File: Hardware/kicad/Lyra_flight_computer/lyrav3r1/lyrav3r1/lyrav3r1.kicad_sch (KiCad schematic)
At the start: 77 parts, among them J1 Conn_01x02, J2 Screw_Terminal_01x06, J3 Conn_01x02, J4 Conn_01x02, J6 Conn_01x06, J7 USB_B_Micro, J8 Conn_01x04, J9 Screw_Terminal_01x06, Q1 AO3401A, Q2 AO3400A, Q3 AO3400A, Q4 AO3400A, Q5 AO3400A, U1 STM32WLE5CBUx, U2 BMI088, U3 BMP388, U4 ADXL375BCCZ-RL7, U5 AMS1117-3.3, U8 RP2040, U9 W25Q128JVS, X2 SX1M12.000M10F30TNN

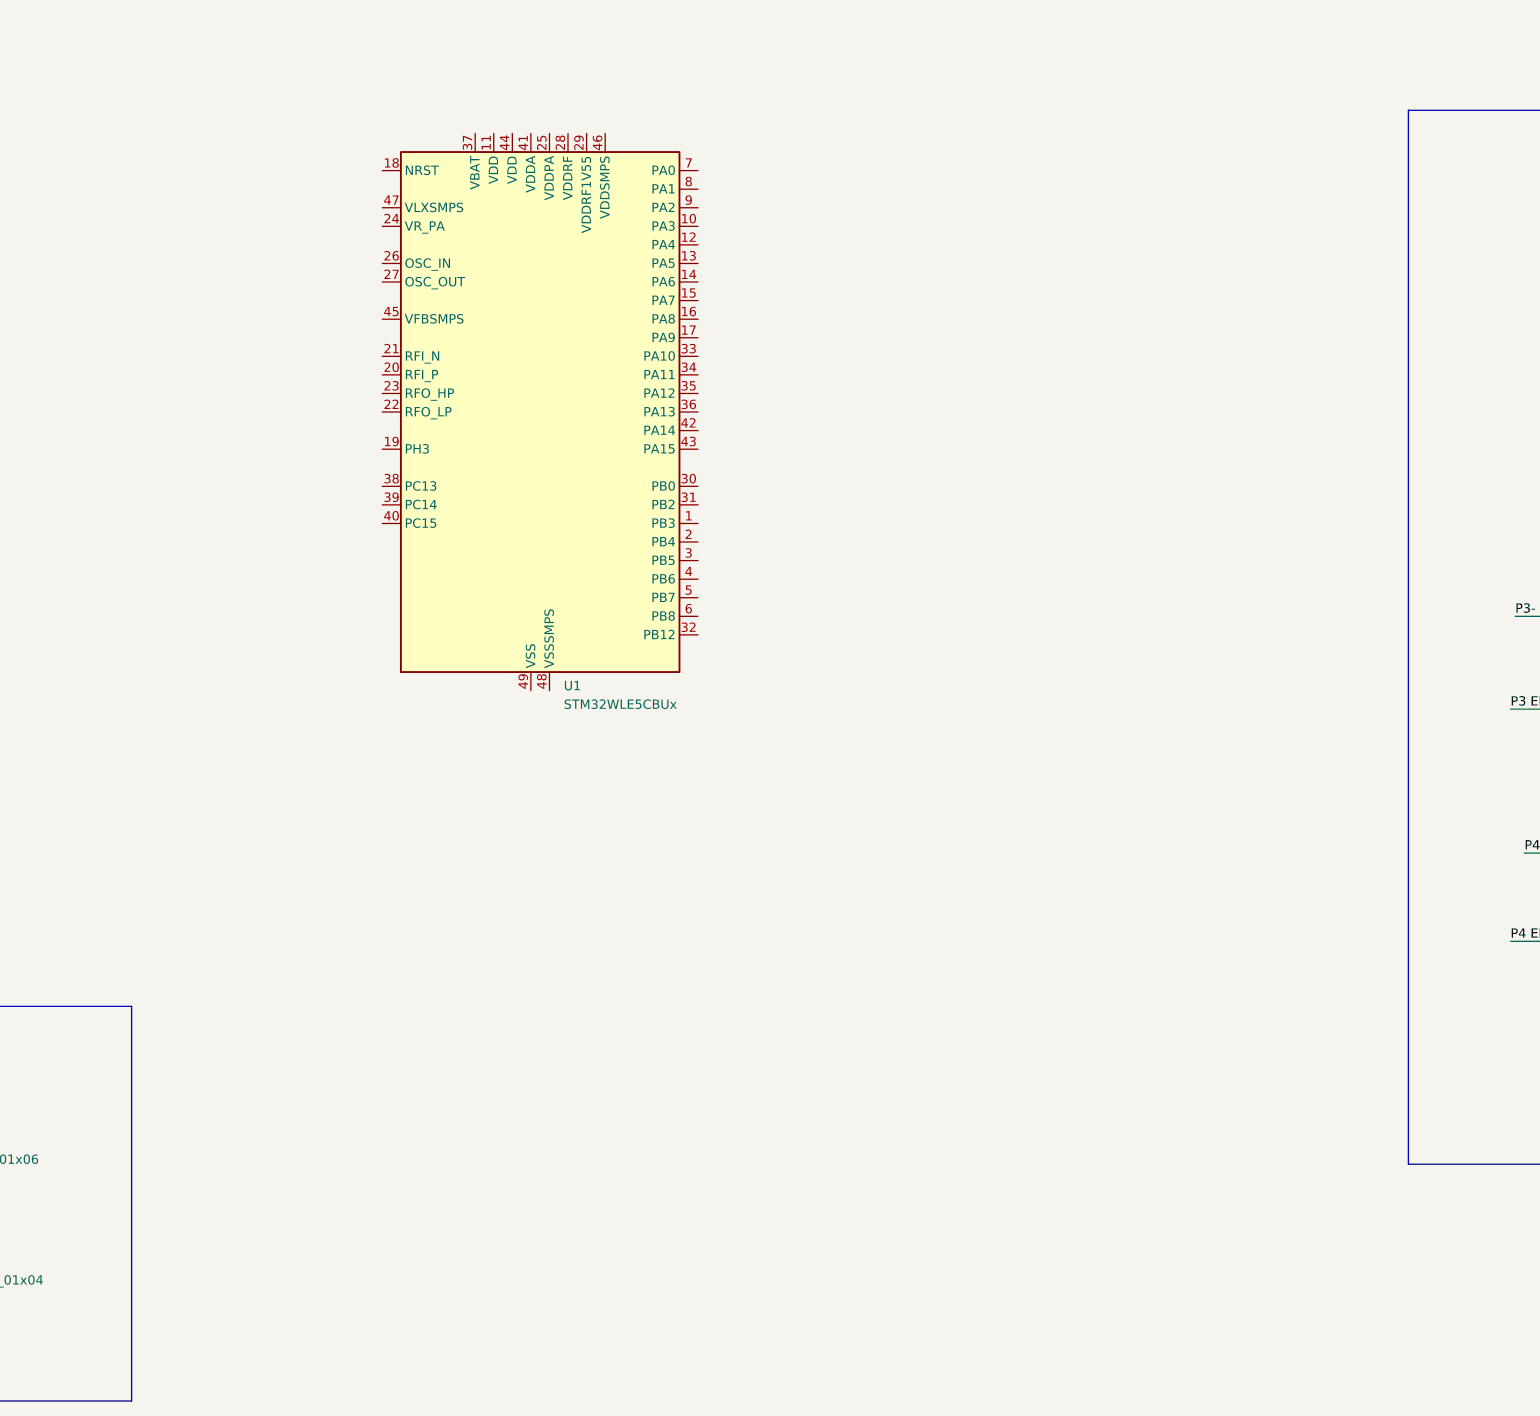
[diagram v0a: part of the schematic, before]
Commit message: stuffs
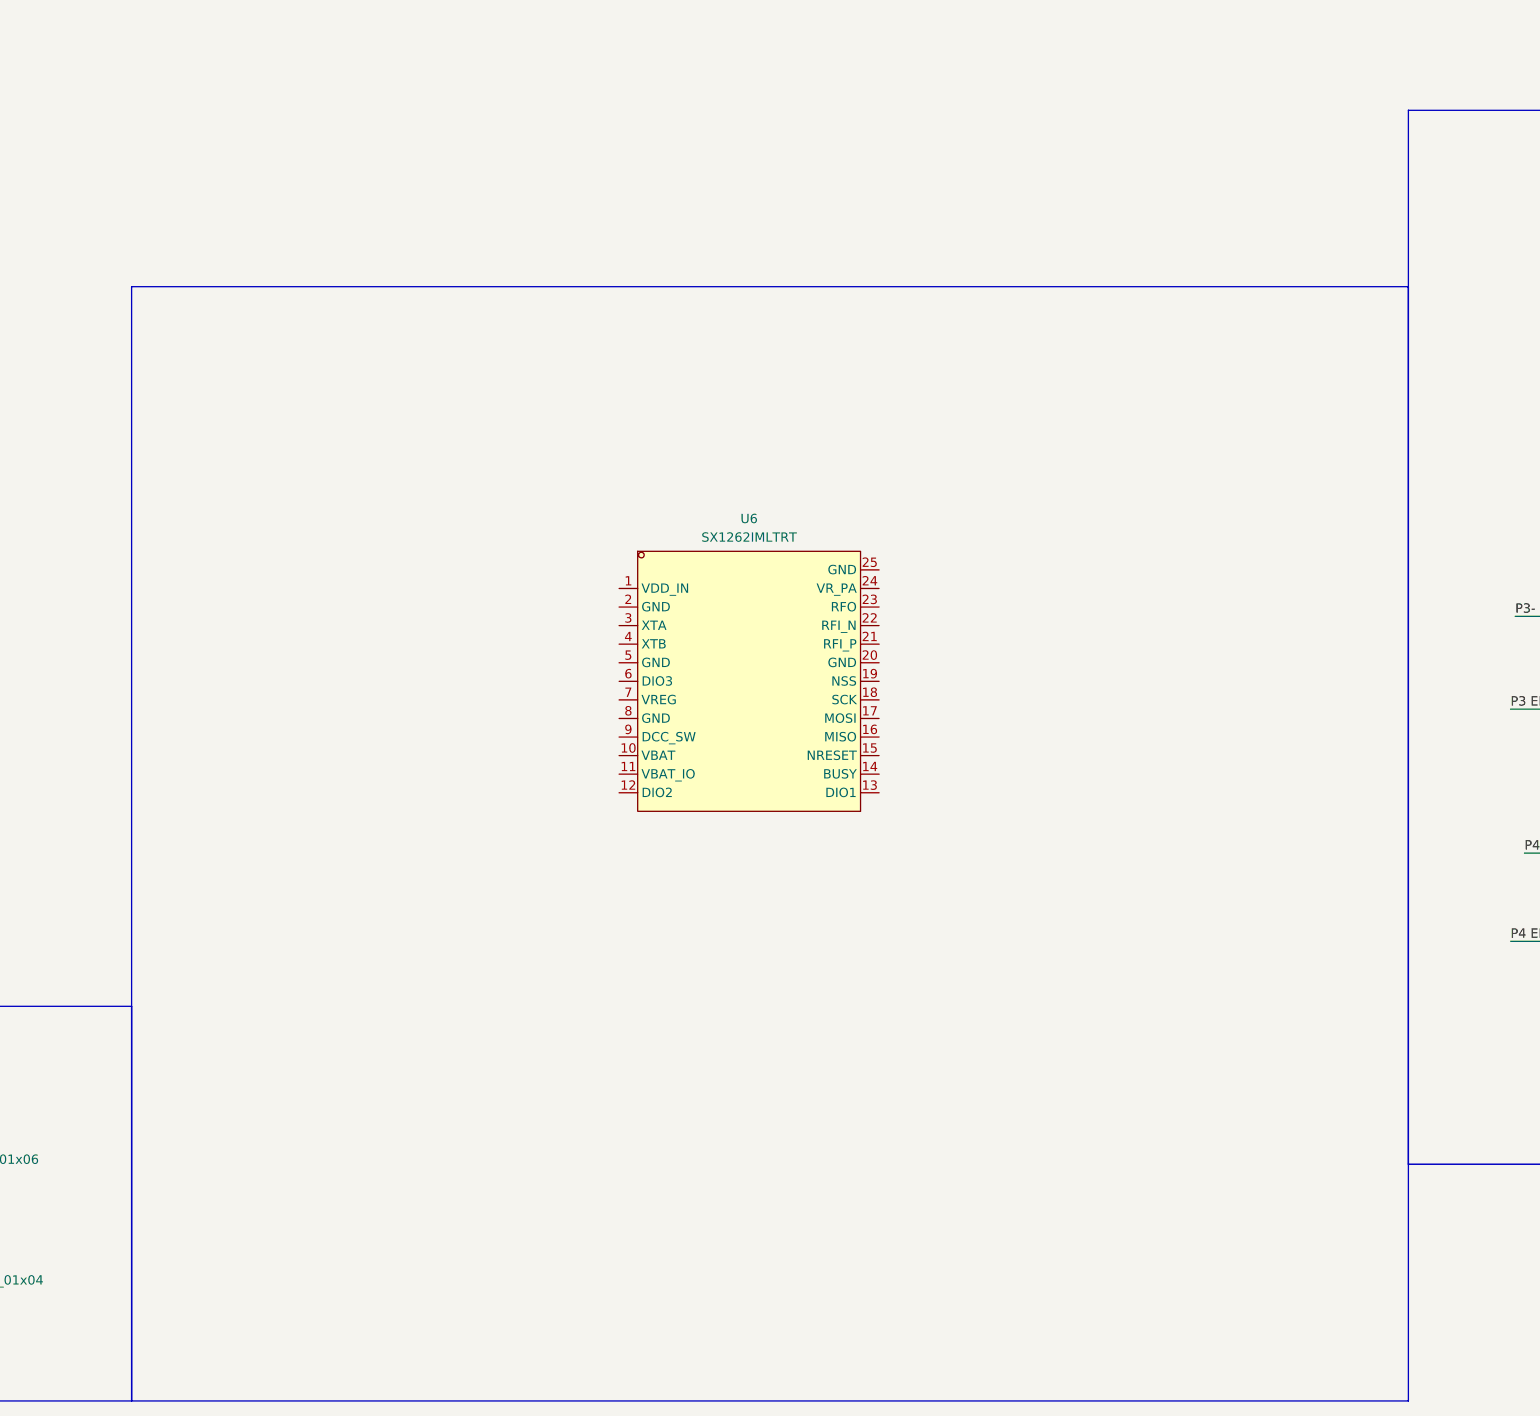
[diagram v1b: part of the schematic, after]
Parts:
- removed U1: STM32WLE5CBUx, Package_DFN_QFN:QFN-48-1EP_7x7mm_P0.5mm_EP5.6x5.6mm, symbol MCU_ST_STM32WL:STM32WLE5CBUx
- added U6: SX1262IMLTRT, easyeda2kicad:QFN-24_L4.0-W4.0-P0.50-BL-EP2.6, symbol easyeda2kicad:SX1262IMLTRT
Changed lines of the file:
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@@
     (fill (type none))
   )
+  (rectangle (start 299.72 255.905) (end 474.345 408.305)
+    (stroke (width 0) (type default))
+    (fill (type none))
+  )
   (rectangle (start 283.845 12.7) (end 407.035 70.485)
     (stroke (width 0) (type default))
@@
     )
   )
+  (symbol (lib_id "easyeda2kicad:SX1262IMLTRT") (at 384.175 309.88 0) (unit 1)
+    (in_bom yes) (on_board yes) (dnp no) (fields_autoplaced)
+    (property "Reference" "U6" (at 384.175 287.655 0)
+      (effects (font (size 1.27 1.27)))
+    )
+    (property "Value" "SX1262IMLTRT" (at 384.175 290.195 0)
+      (effects (font (size 1.27 1.27)))
+    )
+    (property "Footprint" "easyeda2kicad:QFN-24_L4.0-W4.0-P0.50-BL-EP2.6" (at 384.175 332.74 0)
+      (effects (font (size 1.27 1.27)) hide)
+    )
+    (property "Datasheet" "https://lcsc.com/product-detail/Others_STMicroelectronics_SX1262IMLTRT_STMicroelectronics-SX1262IMLTRT_C191341.html" (at 384.175 335.28 0)
+      (effects (font (size 1.27 1.27)) hide)
+    )
+    (property "LCSC Part" "C191341" (at 384.175 337.82 0)
+      (effects (font (size 1.27 1.27)) hide)
+    )
+    (pin "1")
+    (pin "10")
+    (pin "11")
+    (pin "12")
+    (pin "13")
+    (pin "14")
+    (pin "15")
+    (pin "16")
+    (pin "17")
+    (pin "18")
+    (pin "19")
+    (pin "2")
+    (pin "20")
+    (pin "21")
+    (pin "22")
+    (pin "23")
+    (pin "24")
+    (pin "25")
+    (pin "3")
+    (pin "4")
+    (pin "5")
+    (pin "6")
+    (pin "7")
+    (pin "8")
+    (pin "9")
+    (instances
+      (project "lyrav3r1"
+        (path "/12cc3c39-e34e-4801-bd3f-38f875d59424"
+          (reference "U6") (unit 1)
+        )
+      )
+    )
+  )
   (symbol (lib_id "power:GND") (at 554.99 322.58 0) (unit 1)
     (in_bom yes) (on_board yes) (dnp no) (fields_autoplaced)
@@
         )
       )
-    )
-  )
-  (symbol (lib_id "MCU_ST_STM32WL:STM32WLE5CBUx") (at 354.33 273.05 0) (unit 1)
-    (in_bom yes) (on_board yes) (dnp no) (fields_autoplaced)
-    (property "Reference" "U1" (at 358.8259 310.515 0)
-      (effects (font (size 1.27 1.27)) (justify left))
-    )
-    (property "Value" "STM32WLE5CBUx" (at 358.8259 313.055 0)
-      (effects (font (size 1.27 1.27)) (justify left))
-    )
-    (property "Footprint" "Package_DFN_QFN:QFN-48-1EP_7x7mm_P0.5mm_EP5.6x5.6mm" (at 336.55 308.61 0)
-      (effects (font (size 1.27 1.27)) (justify right) hide)
-    )
-    (property "Datasheet" "https://www.st.com/resource/en/datasheet/stm32wle5cb.pdf" (at 354.33 273.05 0)
-      (effects (font (size 1.27 1.27)) hide)
-    )
-    (pin "1")
-    (pin "10")
-    (pin "11")
-    (pin "12")
-    (pin "13")
-    (pin "14")
-    (pin "15")
-    (pin "16")
-    (pin "17")
-    (pin "18")
-    (pin "19")
-    (pin "2")
-    (pin "20")
-    (pin "21")
-    (pin "22")
-    (pin "23")
-    (pin "24")
-    (pin "25")
-    (pin "26")
-    (pin "27")
-    (pin "28")
-    (pin "29")
-    (pin "3")
-    (pin "30")
-    (pin "31")
-    (pin "32")
-    (pin "33")
-    (pin "34")
-    (pin "35")
-    (pin "36")
-    (pin "37")
-    (pin "38")
-    (pin "39")
-    (pin "4")
-    (pin "40")
-    (pin "41")
-    (pin "42")
-    (pin "43")
-    (pin "44")
-    (pin "45")
-    (pin "46")
-    (pin "47")
-    (pin "48")
-    (pin "49")
-    (pin "5")
-    (pin "6")
-    (pin "7")
-    (pin "8")
-    (pin "9")
-    (instances
-      (project "lyrav3r1"
-        (path "/12cc3c39-e34e-4801-bd3f-38f875d59424"
-          (reference "U1") (unit 1)
-        )
-      )

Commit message: asd
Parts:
- removed J6: Conn_01x06, Connector_PinHeader_2.54mm:PinHeader_1x06_P2.54mm_Vertical, symbol Connector_Generic:Conn_01x06
- removed J8: Conn_01x04, Connector_PinHeader_2.54mm:PinHeader_1x04_P2.54mm_Vertical, symbol Connector_Generic:Conn_01x04
- added D3: D, symbol Device:D
- added J5: Conn_01x05, symbol Connector_Generic:Conn_01x05
- added R8: 100, Resistor_SMD:R_0402_1005Metric, symbol Device:R_Small
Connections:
- net BRKOUT1: now also J5.1 (Pin_1)
- net BRKOUT2: now also J5.2 (Pin_2)
- net BRKOUT3: now also J5.3 (Pin_3)
- net BRKOUT4: now also J5.4 (Pin_4)
- net GND: now also D3.2 (A), J5.5 (Pin_5)
- net P3 EN : now also D3.1 (K), R8.2; no longer Q4.1 (G), R17.2
- new net: Q4.1 (G), R17.2, R8.1
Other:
- note added: "GPS"
- note added: "TELEMETRY"
- moved on the sheet: C13, C16, C17, C18, C19, C21, C22, C23, C24, C25, C26, C27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
